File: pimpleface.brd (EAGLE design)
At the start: 107.9 x 129.2 mm, 31 parts, among them J1 B06B-HCMKK, J2 POWERPOLE_POWER45A_DRILL, J3 POWERPOLE_POWER45A_DRILL

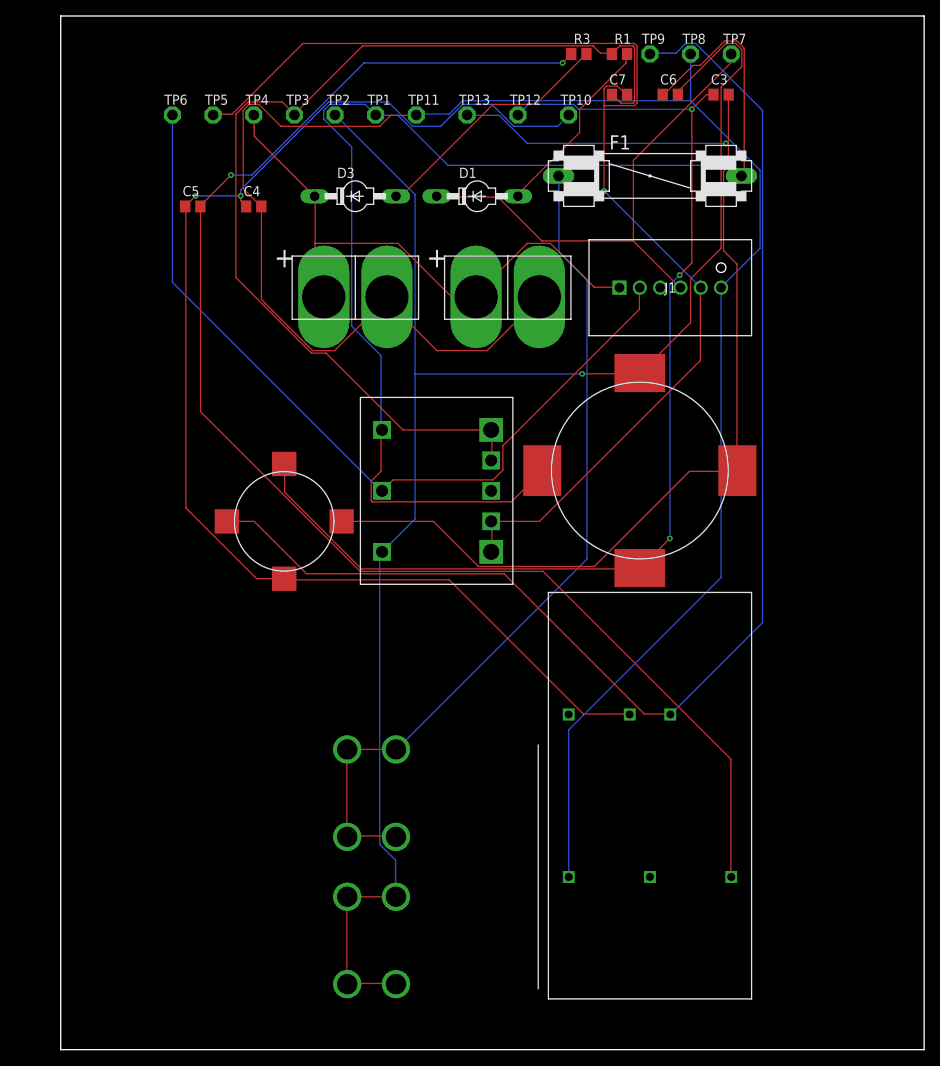
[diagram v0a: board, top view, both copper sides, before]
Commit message: Add files via upload
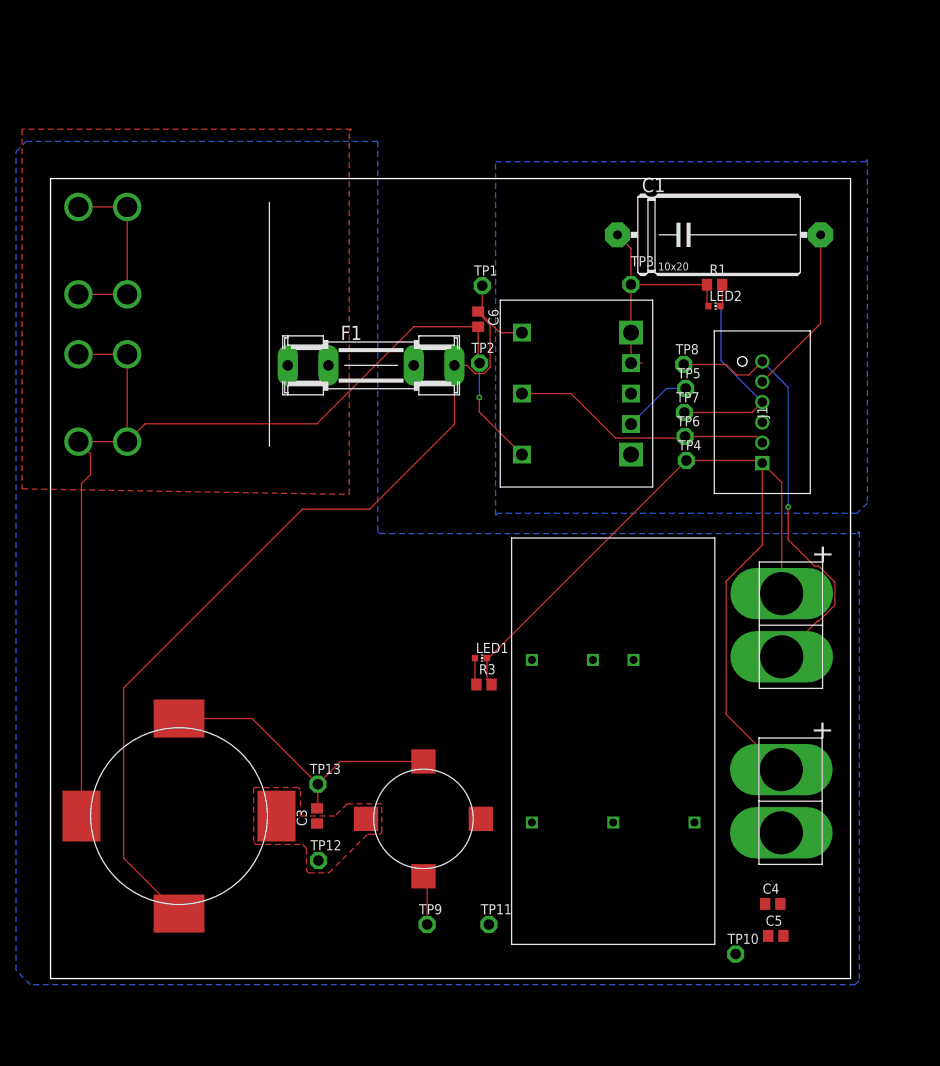
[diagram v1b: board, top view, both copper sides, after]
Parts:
- removed C7: 10uF, rcl:C0805
- removed D1, D3: BYV95, diode:SOD57-10
- added C1: 10uF, rcl:EU25-10
- added LED1, LED2: (no value), led:CHIP-LED0603
- F1: value 7.5A -> FUSESHK20L; device special:FUSE -> fuse:SHK20L
- moved C5 116.7 mm to (90.7, 5.33)
- moved TP9 112.3 mm to (47.1, 6.76)
- moved C4 108.7 mm to (90.3, 9.33)
- moved TP10 106.9 mm to (85.6, 3.06)
- moved C3 103.3 mm to (33.3, 20.3), turned to 90 degrees
- moved TP11 101.6 mm to (54.8, 6.76)
- moved TP12 96.5 mm to (33.5, 14.8)
- moved TP13 85.7 mm to (33.4, 24.3)
- moved J3 84.1 mm to (92.5, 22.2), turned to 270 degrees
- moved R3 79.7 mm to (54.2, 36.8)
- moved U$2 75.7 mm to (9.58, 81.8)
- moved TP6 75.6 mm to (79.3, 67.8)
- moved BUCK150UH 72.0 mm to (16.1, 20.3), turned to 90 degrees
- moved TP4 69.2 mm to (79.5, 64.8)
- moved TP5 68.3 mm to (79.4, 73.8)
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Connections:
- net N$2 renamed TP-12
- net N$5 renamed TP13
- net N$8 renamed 1.6AGND
- removed net JIMGND: C7.2, J1.5, TP5.TP, U$1.-S, U$1.-VOUT
- removed net N$22: D3.C, J1.1, J2.RED, J3.RED, TP4.TP
- removed net N$34: D3.A, R3.2
- removed net N$4: D1.A, R1.2
- removed net N$6: F1.1, U$2.+1, U$2.+2, U$2.+3, U$2.+4
- new net 1.6AOUT: J1.1, J2.RED, J3.RED, LED1.C, R3.2, TP4.TP
- new net 6AGND: C1.2, J1.5, TP5.TP, U$1.-S, U$1.-VOUT
- new net FUSE: F1.1A, U$2.+1, U$2.+2, U$2.+3, U$2.+4
- net LED: now also LED2.C, R1.2; no longer D1.C
- net N$1: now also C1.1, LED2.A; no longer C7.1
- net N$3: now also F1.2A; no longer F1.2
- net N$9: now also LED1.A
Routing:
- net 1.6AGND: track 246.2 -> 56.1 mm, vias 0 -> 1
- net N$9: track 179.0 -> 3.37 mm, vias 2 -> 0
- net N$7: track 163.5 -> 0.00 mm, vias 2 -> 0
- net N$10: track 163.8 -> 6.22 mm
- net JIMGND: track 149.1 -> 0.00 mm, vias 1 -> 0
- net TP-12: track 138.1 -> 0.00 mm, vias 3 -> 0
- net 1.6AOUT: track 0.00 -> 108.7 mm
- net N$6: track 106.4 -> 0.00 mm
- net TP13: track 138.9 -> 38.2 mm, vias 1 -> 0
- net N$1: track 130.1 -> 30.4 mm
- net N$11: track 213.0 -> 139.1 mm
- net N$22: track 72.5 -> 0.00 mm
- net RC: track 104.0 -> 32.8 mm
- net N$3: track 161.3 -> 116.2 mm
- net LED: track 63.7 -> 27.2 mm
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- added copper zone on layer 16, net 1.6AGND
- added copper zone on layer 16, net 6AGND
- added copper zone on layer 1, net FUSE
- added copper zone on layer 1, net TP-12
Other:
- board size 107.9 x 129.2 mm -> 100 x 100 mm
